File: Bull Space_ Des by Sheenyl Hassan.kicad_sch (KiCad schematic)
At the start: 17 parts, among them IC1 TEENSY_4.0, IC2 XB24CZ7PIT-004, J1 Screw_Terminal_01x02, J2 Screw_Terminal_01x02, U1 Regulator_Linear_AP2204RB-3.3, U2 Flight-Computer_Adafruit_GPS_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, U3 ADXL343, U4 BMP280, U6 Memory_Flash_W25Q32JVSS

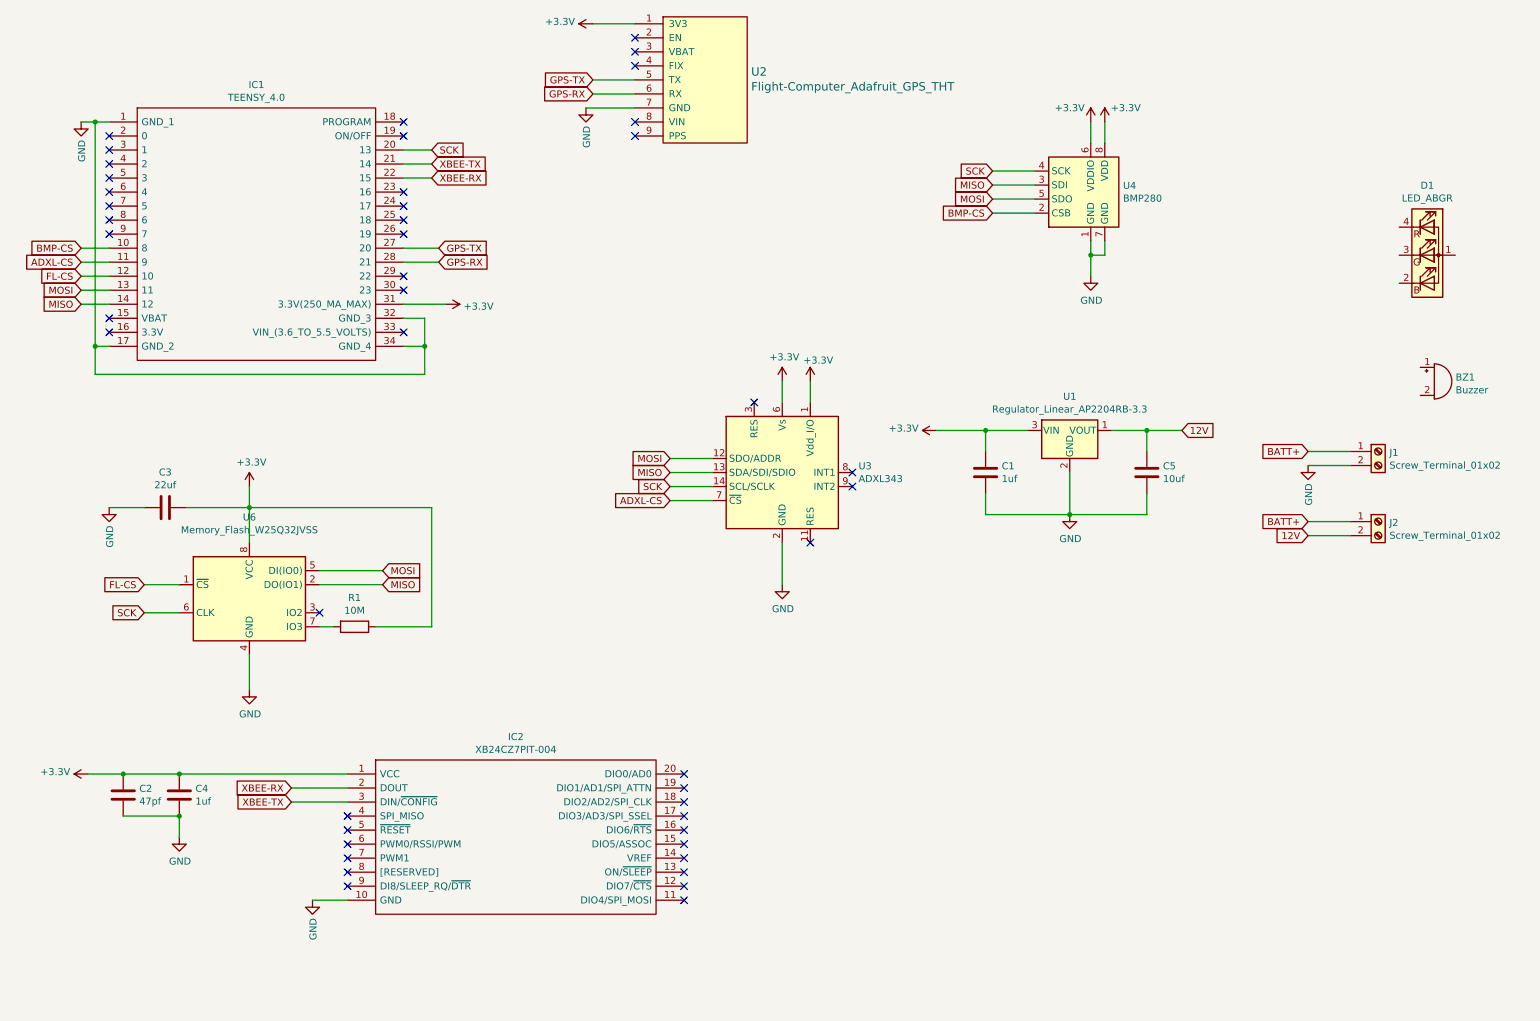
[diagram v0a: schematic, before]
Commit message: Add files via upload
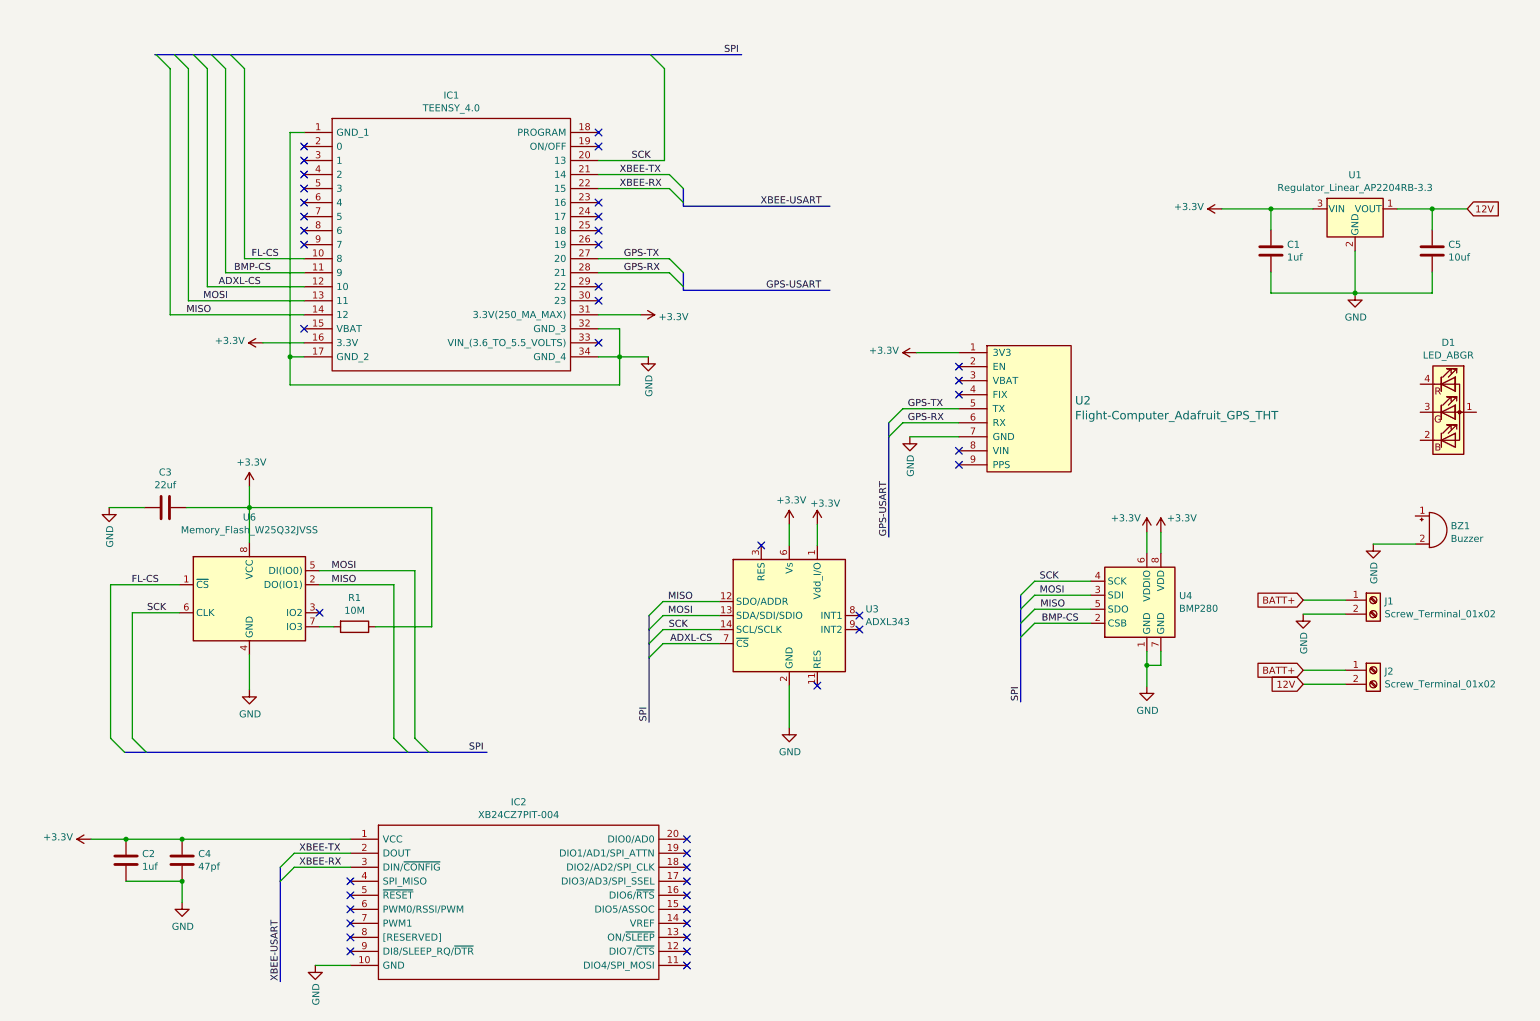
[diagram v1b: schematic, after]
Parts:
- C2: value 47pf -> 1uf
- C4: value 1uf -> 47pf
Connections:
- net +3V3: now also IC1.16 (3.3V)
- net ADXL-CS: now also IC1.12 (10); no longer IC1.11 (9)
- net BMP-CS: now also IC1.11 (9); no longer IC1.10 (8)
- net FL-CS: now also IC1.10 (8); no longer IC1.12 (10)
- net GND: now also BZ1.2 (+)
- net MISO: now also U3.12 (SDO/ADDR), U4.5 (SDO); no longer U3.13 (SDA/SDI/SDIO), U4.3 (SDI)
- net MOSI: now also U3.13 (SDA/SDI/SDIO), U4.3 (SDI); no longer U3.12 (SDO/ADDR), U4.5 (SDO)
- net XBEE-RX: now also IC2.3 (DIN/~{CONFIG}); no longer IC2.2 (DOUT)
- net XBEE-TX: now also IC2.2 (DOUT); no longer IC2.3 (DIN/~{CONFIG})
- no-connect marks 45 -> 44
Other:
- moved on the sheet: BZ1, C1, C2, C4, C5, D1, IC1, IC2, J1, J2, U1, U2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

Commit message: Updates
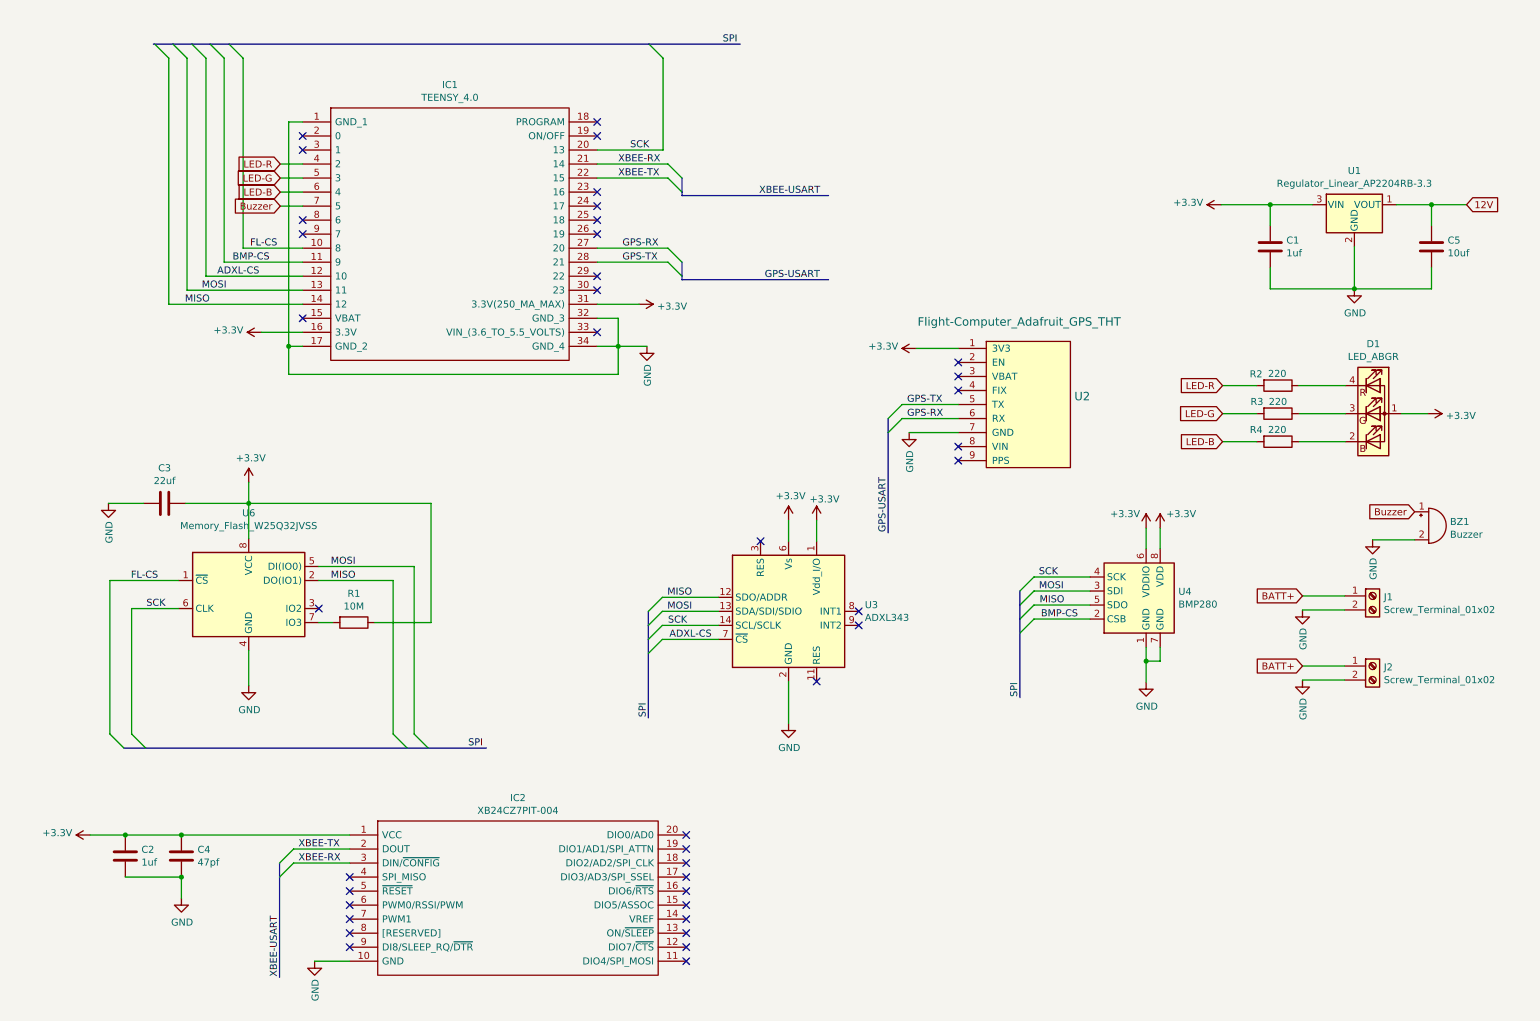
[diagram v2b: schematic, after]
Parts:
- added R2, R3, R4: 220, Resistor_SMD:R_0603_1608Metric_Pad0.98x0.95mm_HandSolder, symbol Device:R
- C1, C5: footprint Capacitor_SMD:C_0603_1608Metric_Pad1.08x0.95mm_HandSolder -> Capacitor_SMD:C_0805_2012Metric_Pad1.18x1.45mm_HandSolder
- C2, C3, C4: footprint (none) -> Capacitor_SMD:C_0805_2012Metric_Pad1.18x1.45mm_HandSolder
- D1: footprint (none) -> LED_THT:LED_D5.0mm-4_RGB_Staggered_Pins
- IC1: footprint TEENSY40 -> Flight Computer:Teensy40
- IC2: footprint XB24CAPIT-001 -> Flight Computer:XBEE_PRO_PTH
- U2: footprint KiCad:Flight-Computer_Adafruit_GPS_THT_Footprint -> Flight Computer:Adafruit_ADXL345_THT
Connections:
- net +3V3: now also D1.1 (A)
- net 12V: no longer J2.2 (Pin_2)
- net GND: now also J2.2 (Pin_2)
- net GPS-RX: now also IC1.27 (20); no longer IC1.28 (21)
- net GPS-TX: now also IC1.28 (21); no longer IC1.27 (20)
- net XBEE-RX: now also IC1.21 (14); no longer IC1.22 (15)
- net XBEE-TX: now also IC1.22 (15); no longer IC1.21 (14)
- net at D1.2 (BK): now also R4.1
- net at D1.3 (GK): now also R3.1
- net at D1.4 (RK): now also R2.1
- net Buzzer: now reaches BZ1.1 (-)
- net Buzzer: now also IC1.7 (5)
- net LED-R: now reaches IC1.4 (2)
- net LED-R: now also R2.2
- net LED-G: now reaches IC1.5 (3)
- net LED-G: now also R3.2
- net LED-B: now reaches IC1.6 (4)
- net LED-B: now also R4.2
- no-connect marks 44 -> 40
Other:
- moved on the sheet: BZ1, C1, C2, C3, C4, C5, D1, IC1, IC2, J1, J2, R1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
